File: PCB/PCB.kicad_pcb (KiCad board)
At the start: 2 copper layers, 11 parts, among them J1 GPIO/Control, J2 POWER

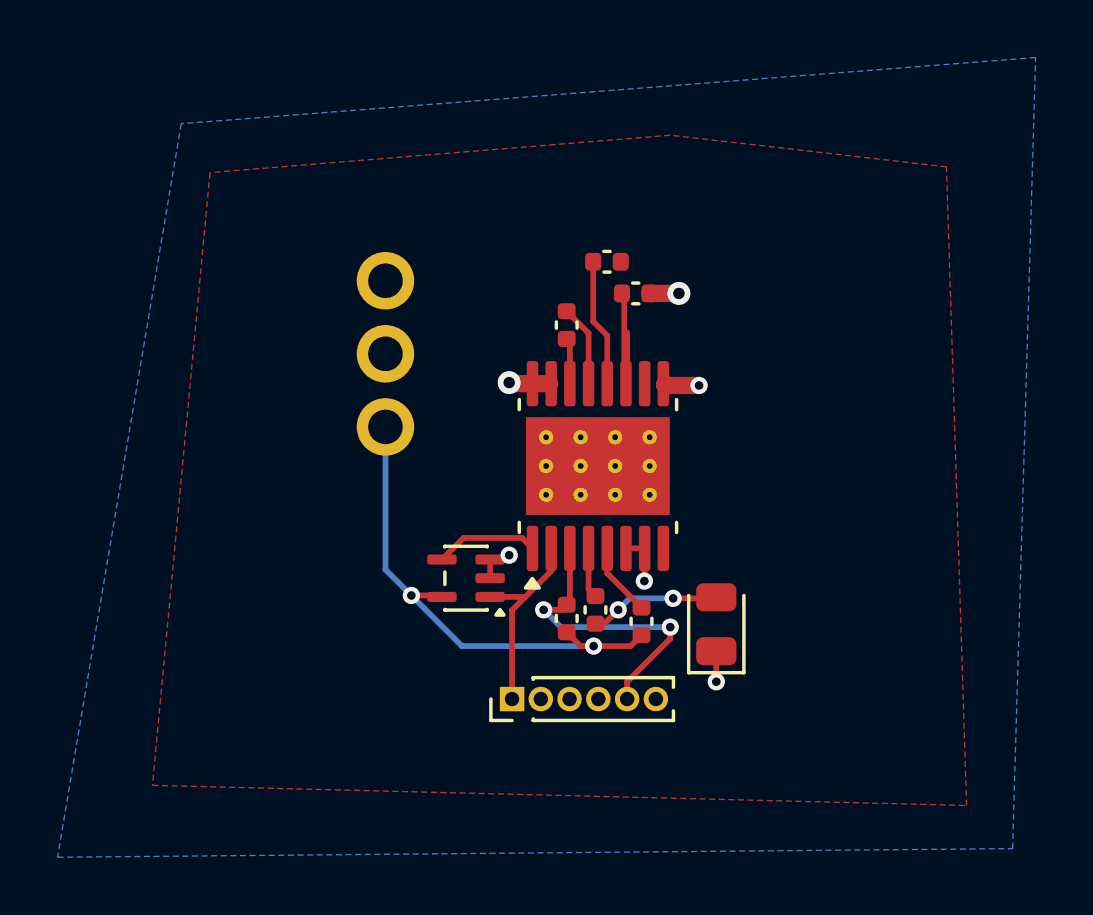
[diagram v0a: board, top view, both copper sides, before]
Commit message: commite
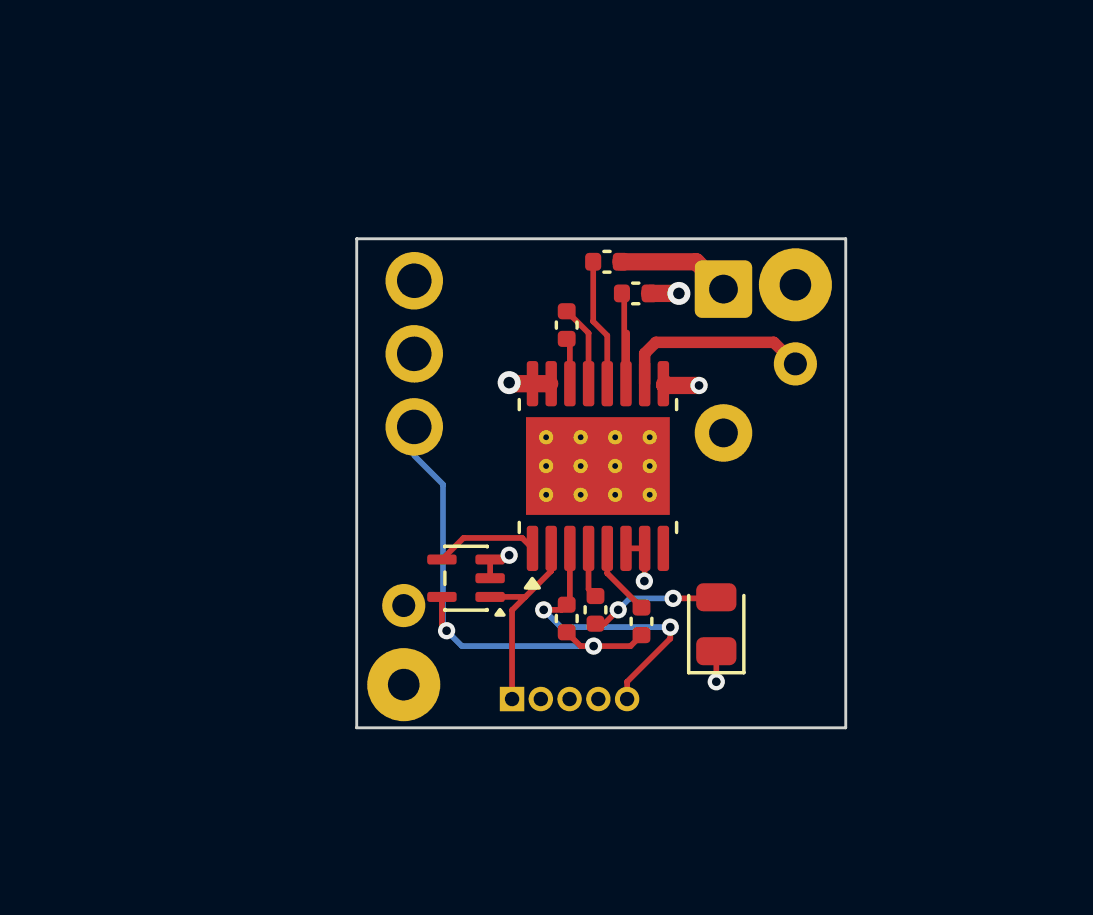
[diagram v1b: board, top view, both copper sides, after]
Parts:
- added C2: 22uf, Capacitor_THT:CP_Radial_D10.0mm_P5.00mm, B.Cu at (108.8, 96.8)
- added J3: OUTPUT2, Taranium-libs:Electromagnet Power Output, F.Cu at (111.2, 96.6)
- added J4: OUTPUT1, Taranium-libs:Electromagnet Power Output, F.Cu at (97.6, 110.5)
- J1: footprint Connector_PinHeader_1.00mm:PinHeader_1x06_P1.00mm_Vertical -> Connector_PinHeader_1.00mm:PinHeader_1x05_P1.00mm_Vertical; moved to B.Cu
- moved J2 1.00 mm to (98.0, 99.0)
- turned J1 to -90 degrees
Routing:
- net /OUT2: track 0.00 -> 6.76 mm
- net +24V: track 4.74 -> 8.71 mm
- net +3V3: track 17.3 -> 16.1 mm
- removed copper zone on F.Cu, net +24V
- removed copper zone on B.Cu, net GND
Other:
- board outline added: 17 x 17 mm
